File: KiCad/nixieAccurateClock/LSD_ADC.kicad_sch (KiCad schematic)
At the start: 13 parts, among them U10 TXB0108DQSR, U11 TXB0108DQSR

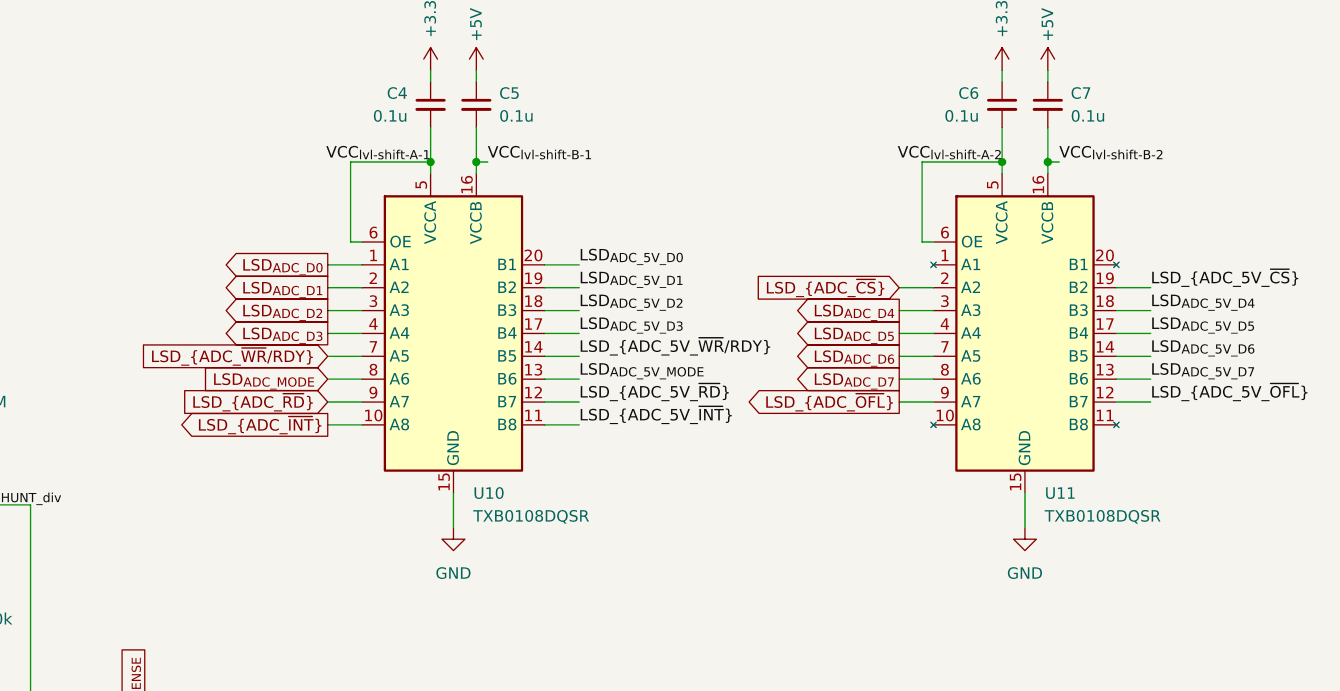
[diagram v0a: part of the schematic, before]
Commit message: Switch to <6 mil package for level shifting
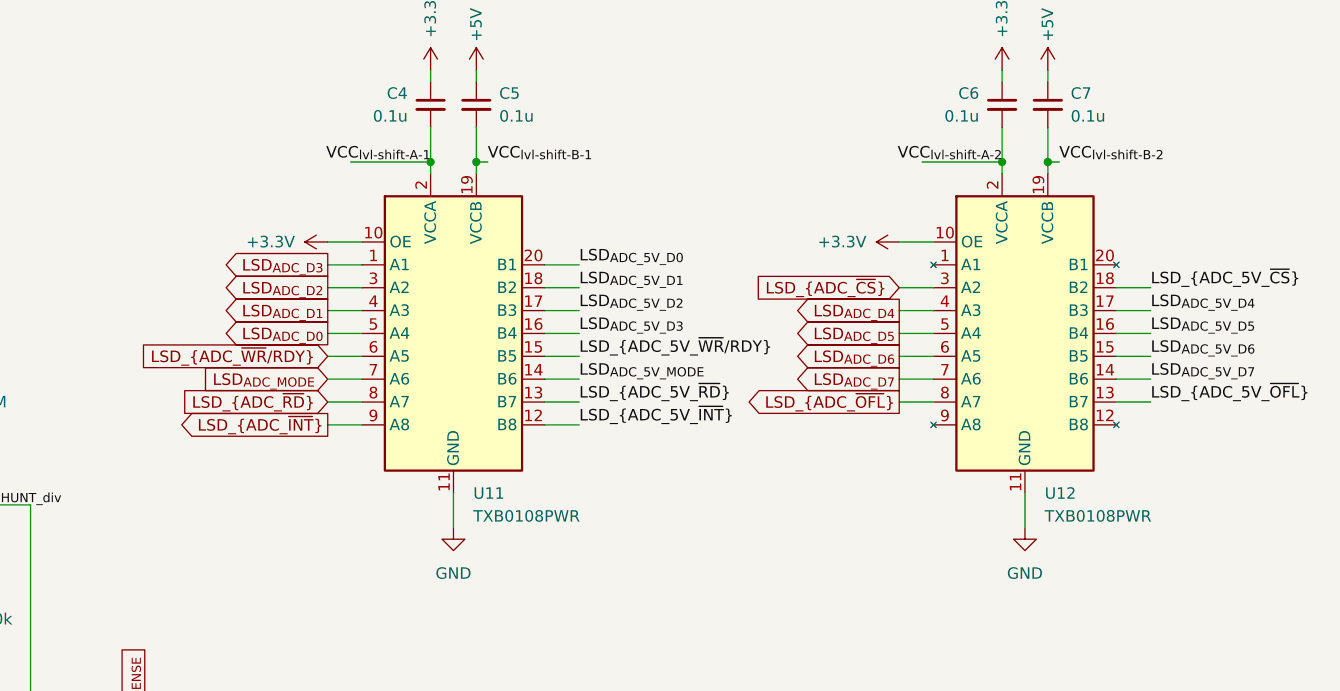
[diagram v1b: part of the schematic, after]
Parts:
- removed U10, U11: TXB0108DQSR, Package_SON:USON-20_2x4mm_P0.4mm, symbol Logic_LevelTranslator:TXB0108DQSR
- added U11, U12: TXB0108PWR, Package_SO:TSSOP-20_4.4x6.5mm_P0.65mm, symbol 00_lib:TXB0108PWR
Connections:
- net +3.3V: now also U11.10 (OE), U12.10 (OE)
- net GND: now also U11.11 (GND), U12.11 (GND)
- net LSD_{ADC_5V_D0}: now also U11.20 (B1)
- net LSD_{ADC_5V_D1}: now also U11.18 (B2)
- net LSD_{ADC_5V_D2}: now also U11.17 (B3)
- net LSD_{ADC_5V_D3}: now also U11.16 (B4)
- net LSD_{ADC_5V_D4}: now also U12.17 (B3)
- net LSD_{ADC_5V_D5}: now also U12.16 (B4)
- net LSD_{ADC_5V_D6}: now also U12.15 (B5)
- net LSD_{ADC_5V_D7}: now also U12.14 (B6)
- net LSD_{ADC_5V_MODE}: now also U11.14 (B6)
- net LSD_{ADC_5V_~{CS}}: now also U12.18 (B2)
- net LSD_{ADC_5V_~{INT}}: now also U11.12 (B8)
- net LSD_{ADC_5V_~{OFL}}: now also U12.13 (B7)
- net LSD_{ADC_5V_~{RD}}: now also U11.13 (B7)
- net LSD_{ADC_5V_~{WR}/RDY}: now also U11.15 (B5)
- net LSD_{ADC_D0}: now also U11.5 (A4)
- net LSD_{ADC_D1}: now also U11.4 (A3)
- net LSD_{ADC_D2}: now also U11.3 (A2)
- net LSD_{ADC_D3}: now also U11.1 (A1)
- net LSD_{ADC_D4}: now also U12.4 (A3)
- net LSD_{ADC_D5}: now also U12.5 (A4)
- net LSD_{ADC_D6}: now also U12.6 (A5)
- net LSD_{ADC_D7}: now also U12.7 (A6)
- net LSD_{ADC_MODE}: now also U11.7 (A6)
- net LSD_{ADC_~{CS}}: now also U12.3 (A2)
- net LSD_{ADC_~{INT}}: now also U11.9 (A8)
- net LSD_{ADC_~{OFL}}: now also U12.8 (A7)
- net LSD_{ADC_~{RD}}: now also U11.8 (A7)
- net LSD_{ADC_~{WR}/RDY}: now also U11.6 (A5)
- net VCC_{lvl-shift-A-1}: now also U11.2 (VCCA)
- net VCC_{lvl-shift-A-2}: now also U12.2 (VCCA)
- net VCC_{lvl-shift-B-1}: now also U11.19 (VCCB)
- net VCC_{lvl-shift-B-2}: now also U12.19 (VCCB)
